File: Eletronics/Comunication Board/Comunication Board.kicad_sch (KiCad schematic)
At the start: 29 parts, among them K1 RELE, T1 AMS1117/3V3, U1 ESP32-S3-WROOM-1-N8R2, U2 BATERIA, U3 MAX17048G

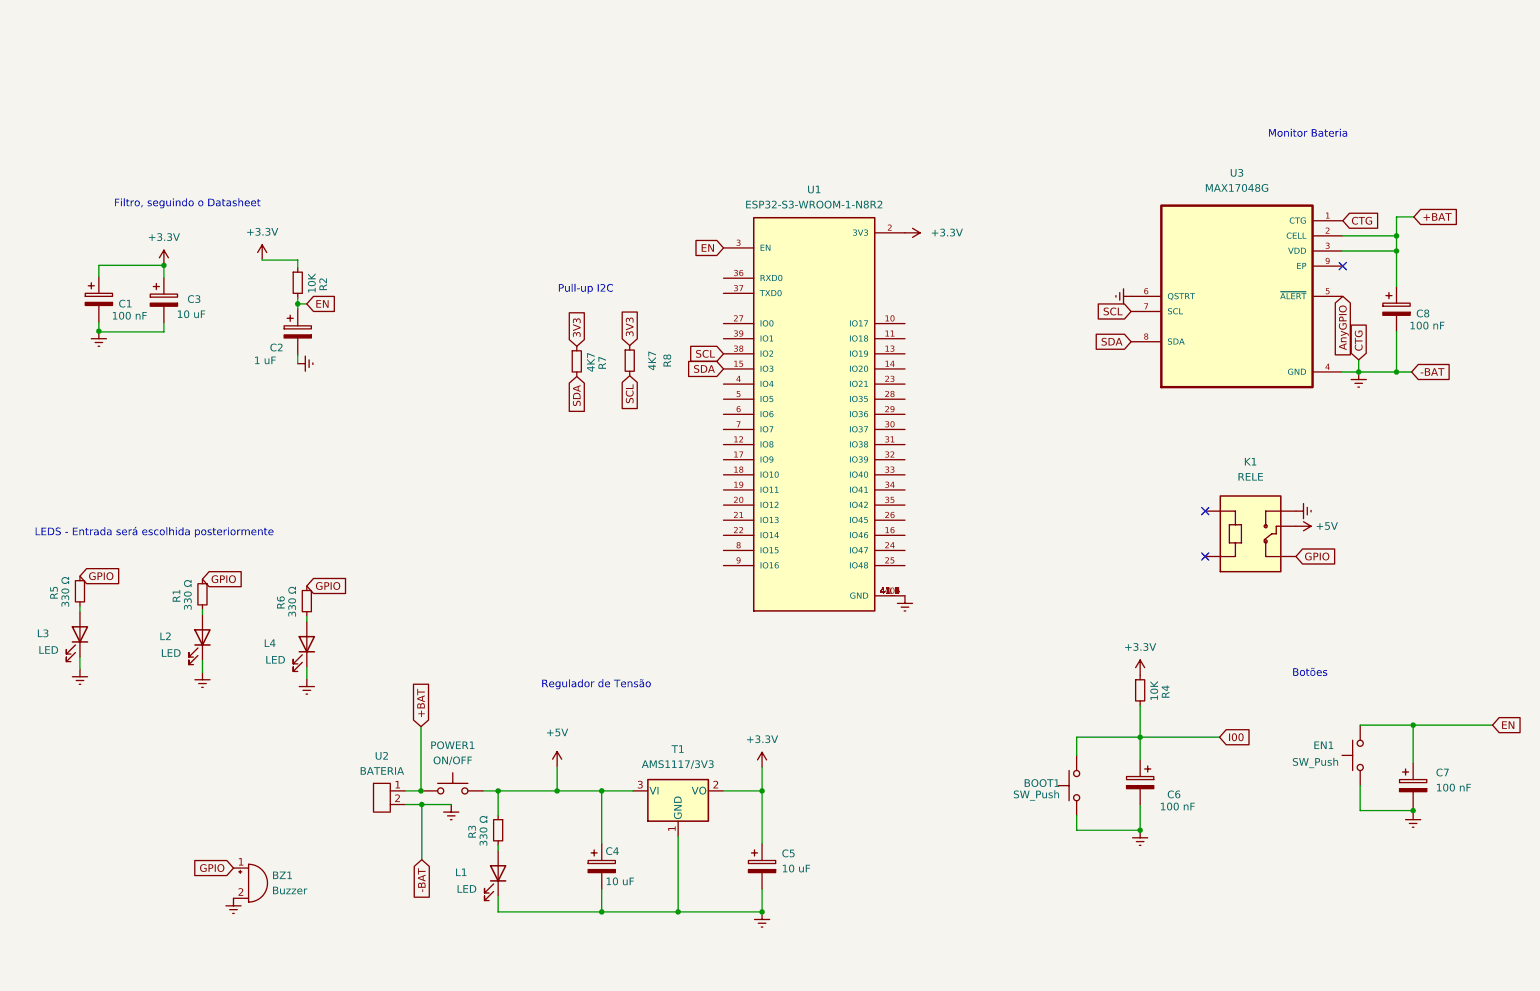
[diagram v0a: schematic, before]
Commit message: Comunication Board edit
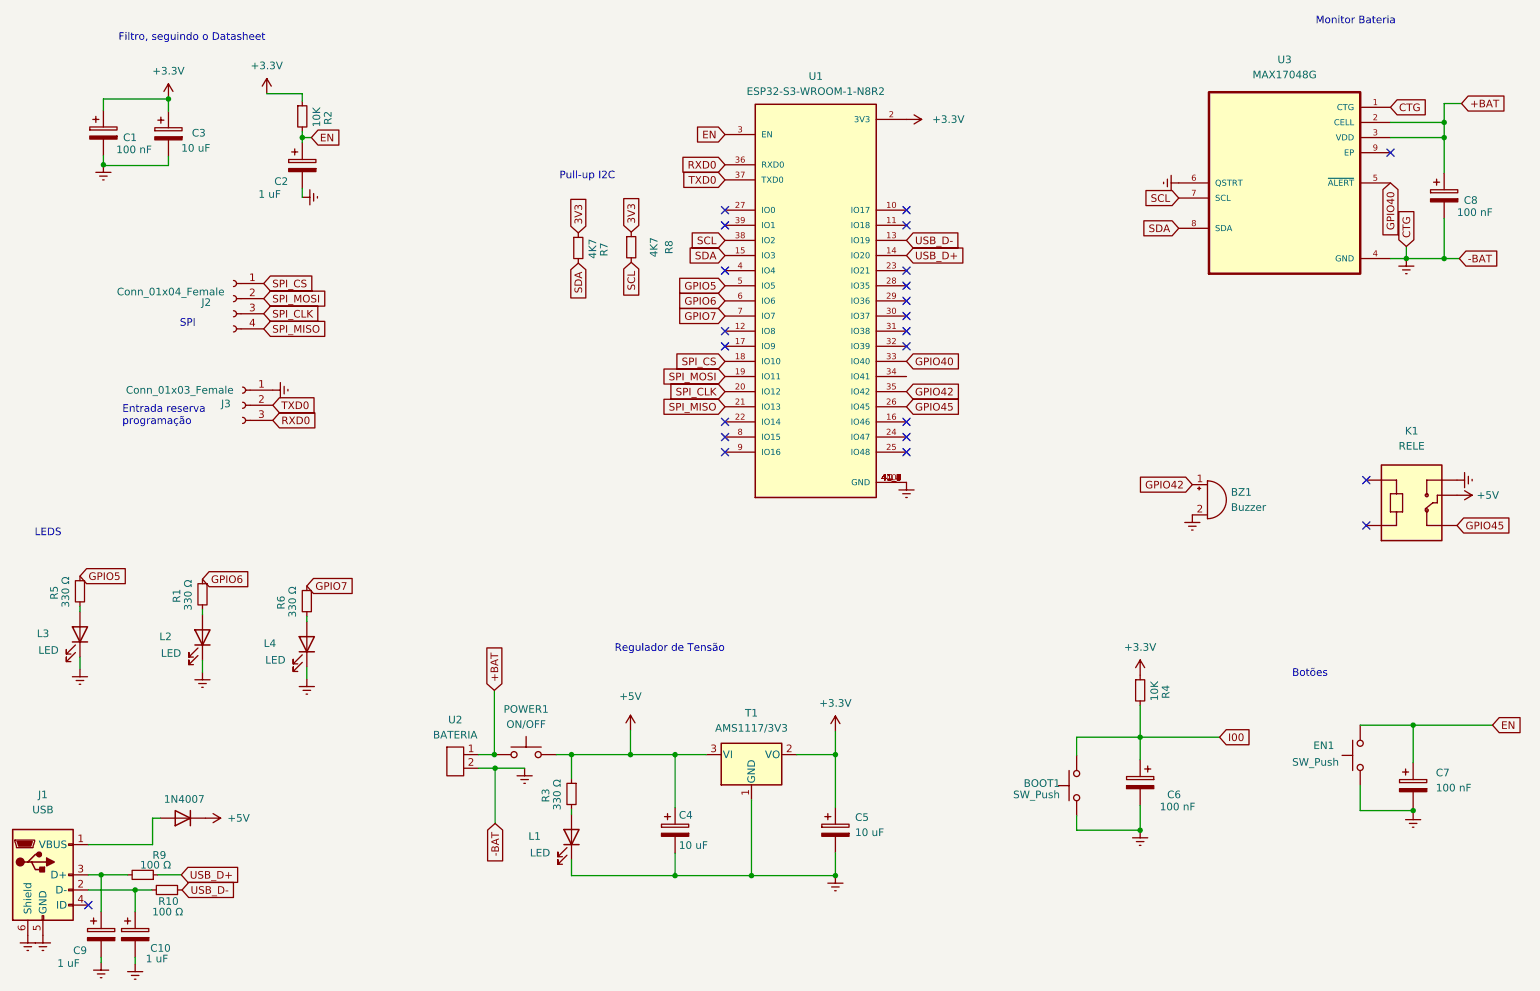
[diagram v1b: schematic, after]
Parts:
- added C10, C9: 1 uF, Capacitor_SMD:C_0603_1608Metric, symbol Device:C_Polarized
- added D1: 1N4007, Diode_SMD:D_SMA, symbol Diode:1N4007
- added J1: USB, Connector_USB:USB_Micro-B_Amphenol_10118194_Horizontal, symbol Connector:USB_B_Micro
- added J2: Conn_01x04_Female, symbol Connector:Conn_01x04_Female
- added J3: Conn_01x03_Female, Connector_PinSocket_2.54mm:PinSocket_1x03_P2.54mm_Vertical, symbol Connector:Conn_01x03_Female
- added R10, R9: 100 Ω, Resistor_SMD:R_0603_1608Metric, symbol Device:R_Small
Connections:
- net AnyGPIO is gone; now on net GPIO40: U3.5 (~{ALERT})
- net +5V: now also D1.1 (K)
- net GNDREF: now also C10.2, C9.2, J1.5 (GND), J1.6 (Shield), J3.1 (Pin_1)
- net USB_D-: now reaches U1.13 (IO19)
- net USB_D-: now also R10.1
- net USB_D+: now reaches U1.14 (IO20)
- net USB_D+: now also R9.1
- net SPI_CS: now reaches U1.18 (IO10)
- net SPI_CS: now also J2.1 (Pin_1)
- net SPI_MOSI: now reaches U1.19 (IO11)
- net SPI_MOSI: now also J2.2 (Pin_2)
- net SPI_CLK: now reaches U1.20 (IO12)
- net SPI_CLK: now also J2.3 (Pin_3)
- net SPI_MISO: now reaches U1.21 (IO13)
- net SPI_MISO: now also J2.4 (Pin_4)
- net GPIO45: now reaches U1.26 (IO45)
- net GPIO45: now also K1.NC
- net GPIO40: now reaches U1.33 (IO40)
- net GPIO42: now reaches U1.35 (IO42)
- net GPIO42: now also BZ1.1 (-)
- net RXD0: now reaches U1.36 (RXD0)
- net RXD0: now also J3.3 (Pin_3)
- net TXD0: now reaches U1.37 (TXD0)
- net TXD0: now also J3.2 (Pin_2)
- net GPIO5: now reaches U1.5 (IO5)
- net GPIO5: now also R5.1
- net GPIO6: now reaches U1.6 (IO6)
- net GPIO6: now also R1.1
- net GPIO7: now reaches U1.7 (IO7)
- net GPIO7: now also R6.1
- removed net GPIO: BZ1.1 (-), K1.NC, R1.1, R5.1, R6.1
- new net: C10.1, J1.2 (D-), R10.2
- new net: D1.2 (A), J1.1 (VBUS)
- new net: C9.1, J1.3 (D+), R9.2
- no-connect marks 3 -> 23
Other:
- note added: "Entrada reserva programação"
- note added: "LEDS"
- note added: "SPI"
- note removed: "LEDS - Entrada será escolhida posteriormente"
- moved on the sheet: BZ1, C1, C2, C3, C4, C5, C8, K1, L1, POWER1, R2, R3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
